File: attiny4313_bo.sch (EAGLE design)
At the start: 11 parts, among them J1 AVR_SPI_PRG_6NS, Y1 16MHz

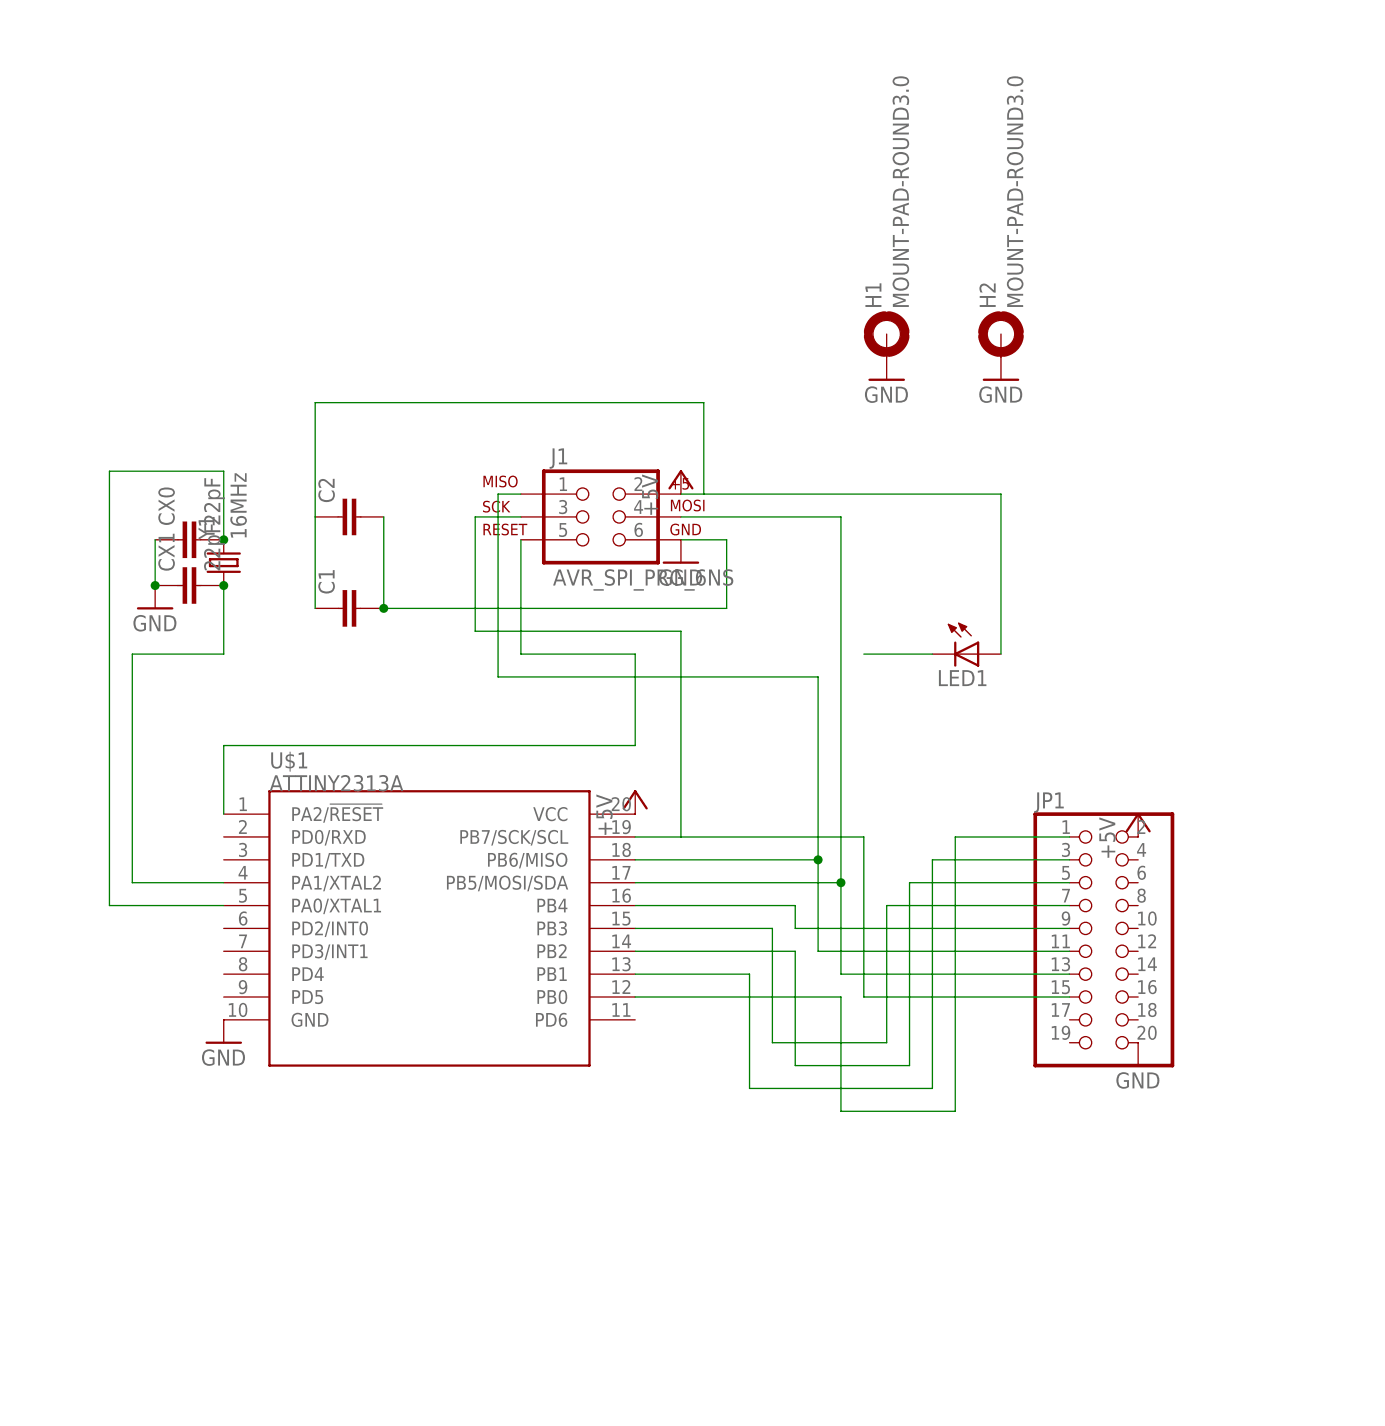
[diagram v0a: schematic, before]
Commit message: signals v1, probably bad
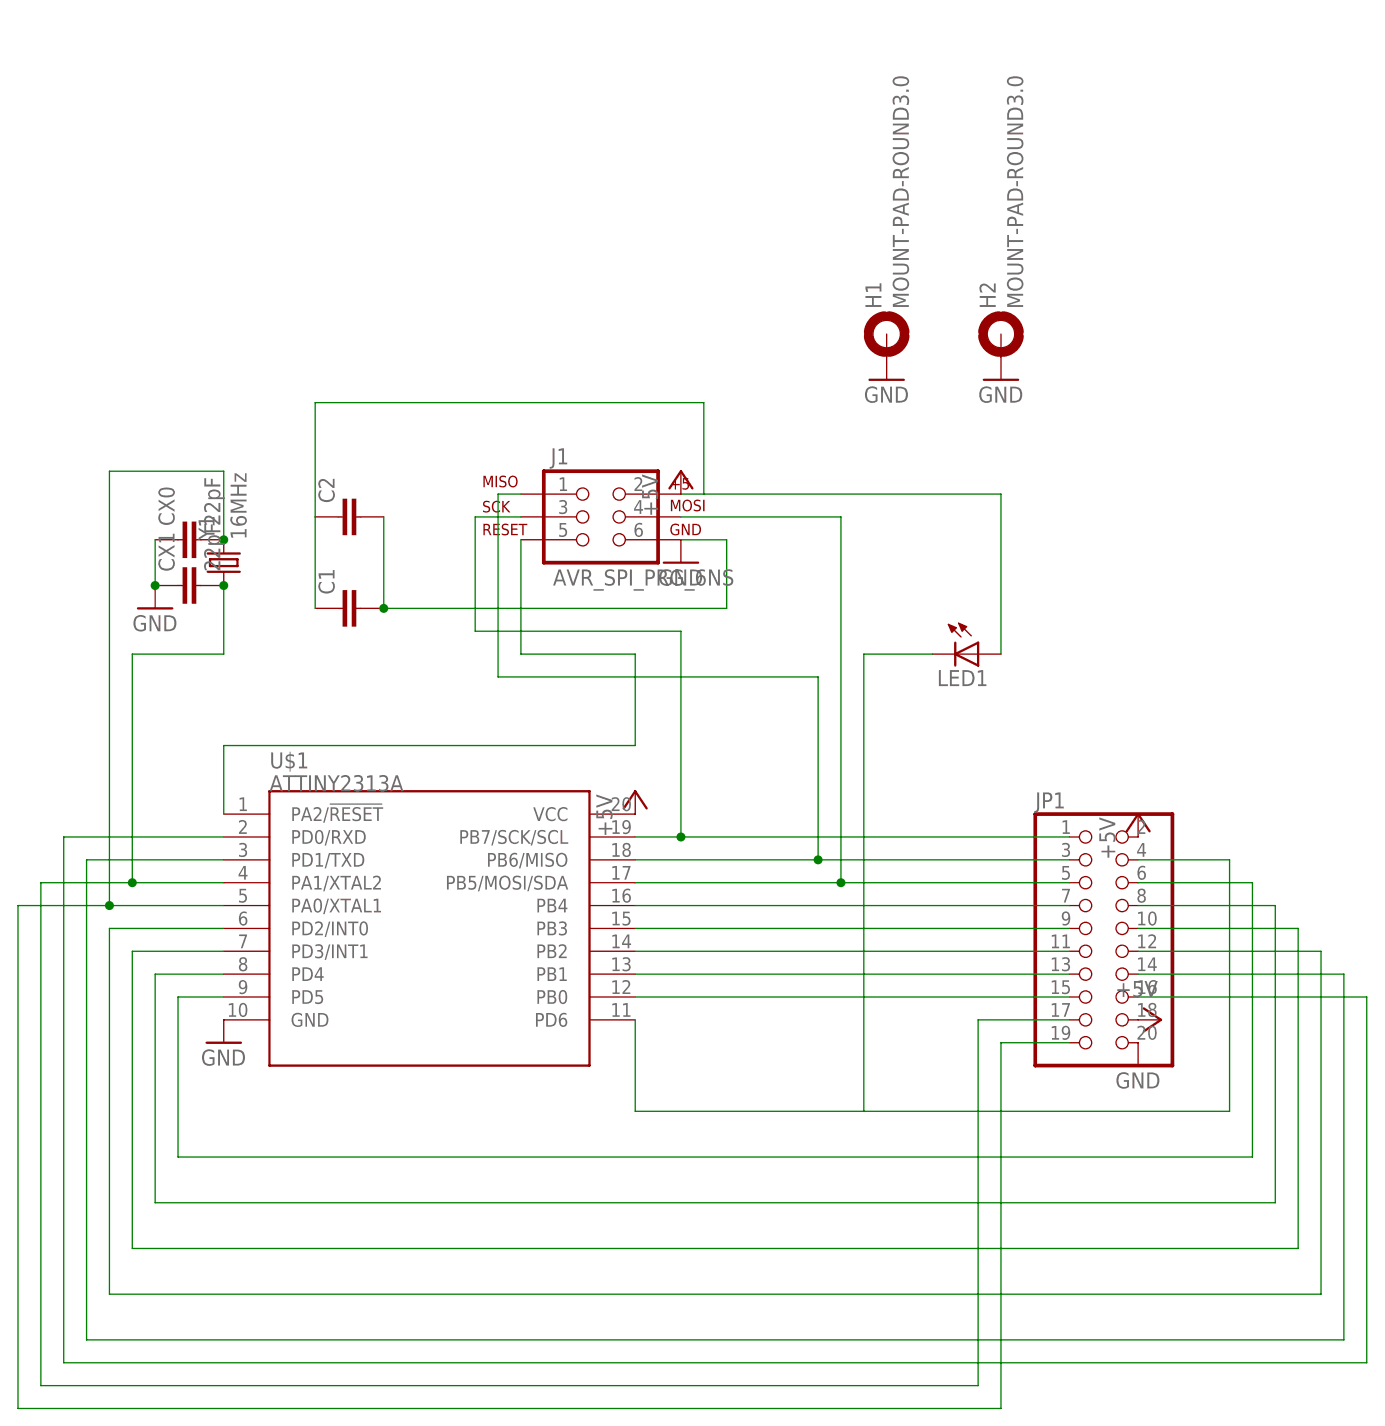
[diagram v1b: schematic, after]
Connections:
- removed net N$1: CX0.2, U$1.PA0/XTAL1, Y1.2
- removed net N$2: LED1.C
- removed net PB0/XTAL1: CX1.2, U$1.PA1/XTAL2, Y1.1
- new net PA0/XTAL1: CX0.2, JP1.19, U$1.PA0/XTAL1, Y1.2
- new net PA1/XTAL2: CX1.2, JP1.17, U$1.PA1/XTAL2, Y1.1
- new net PD0/RDX: JP1.16, U$1.PD0/RXD
- new net PD1/TXD: JP1.14, U$1.PD1/TXD
- new net PD2: JP1.12, U$1.PD2/INT0
- new net PD3: JP1.10, U$1.PD3/INT1
- new net PD4: JP1.8, U$1.PD4
- new net PD5: JP1.6, U$1.PD5
- new net PD6: JP1.4, LED1.C, U$1.PD6
- net +5V: now also JP1.18
- net PB0: now also JP1.15; no longer JP1.1
- net PB1: now also JP1.13; no longer JP1.3
- net PB2: now also JP1.11; no longer JP1.5
- net PB3: now also JP1.9; no longer JP1.7
- net PB4: now also JP1.7; no longer JP1.9
- net PB5/MOSI: now also JP1.5; no longer JP1.13
- net PB6/MISO: now also JP1.3; no longer JP1.11
- net PB7/SCL: now also JP1.1; no longer JP1.15

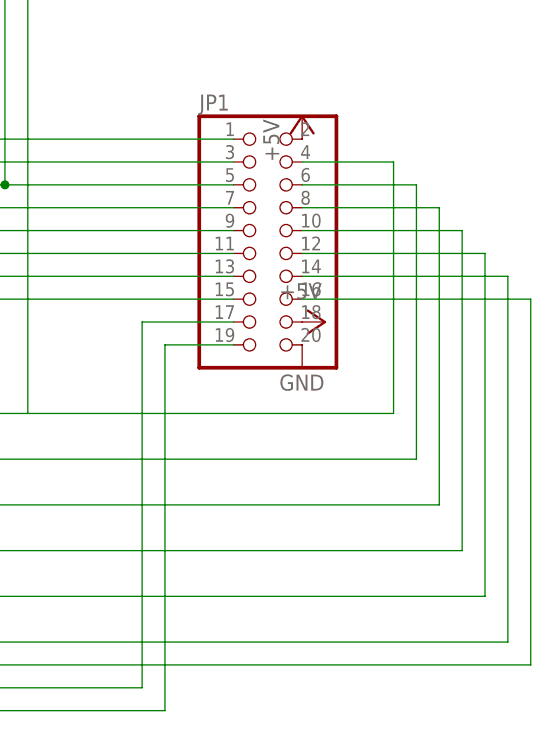
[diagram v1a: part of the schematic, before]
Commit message: pin identifiers
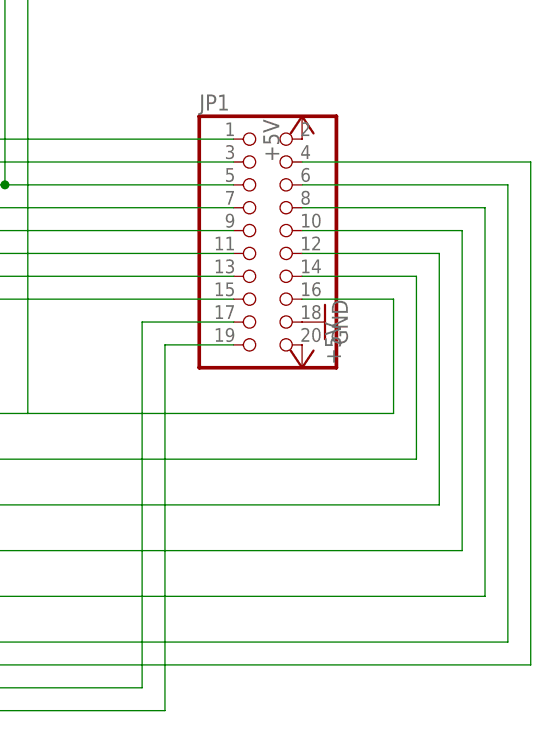
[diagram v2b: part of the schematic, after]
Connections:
- net +5V: now also JP1.20; no longer JP1.18
- net GND: now also JP1.18; no longer JP1.20
- net PD0/RDX: now also JP1.4; no longer JP1.16
- net PD1/TXD: now also JP1.6; no longer JP1.14
- net PD2: now also JP1.8; no longer JP1.12
- net PD4: now also JP1.12; no longer JP1.8
- net PD5: now also JP1.14; no longer JP1.6
- net PD6: now also JP1.16; no longer JP1.4
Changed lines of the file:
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@@
 <part name="P+2" library="supply1" deviceset="+5V" device=""/>
 <part name="JP1" library="pinhead" deviceset="PINHD-2X10" device=""/>
+<part name="P+3" library="supply1" deviceset="+5V" device=""/>
 <part name="GND2" library="supply1" deviceset="GND" device=""/>
-<part name="P+3" library="supply1" deviceset="+5V" device=""/>
 </parts>
 <sheets>
@@
 <instance part="P+2" gate="1" x="127" y="73.66"/>
 <instance part="JP1" gate="A" x="121.92" y="60.96"/>
-<instance part="GND2" gate="1" x="127" y="45.72"/>
-<instance part="P+3" gate="1" x="129.54" y="50.8" rot="R270"/>
+<instance part="P+3" gate="1" x="127" y="45.72" rot="R180"/>
+<instance part="GND2" gate="1" x="129.54" y="50.8" rot="R90"/>
 </instances>
 <busses>
@@
 </segment>
 <segment>
-<pinref part="JP1" gate="A" pin="20"/>
+<pinref part="JP1" gate="A" pin="18"/>
 <pinref part="GND2" gate="1" pin="GND"/>
 </segment>
@@
 </segment>
 <segment>
-<pinref part="JP1" gate="A" pin="18"/>
+<pinref part="JP1" gate="A" pin="20"/>
 <pinref part="P+3" gate="1" pin="+5V"/>
 </segment>
@@
 <segment>
 <wire x1="7.62" y1="12.7" x2="152.4" y2="12.7" width="0.1524" layer="91"/>
-<wire x1="152.4" y1="12.7" x2="152.4" y2="53.34" width="0.1524" layer="91"/>
-<pinref part="JP1" gate="A" pin="16"/>
-<wire x1="152.4" y1="53.34" x2="127" y2="53.34" width="0.1524" layer="91"/>
+<wire x1="152.4" y1="12.7" x2="152.4" y2="68.58" width="0.1524" layer="91"/>
 <wire x1="7.62" y1="12.7" x2="7.62" y2="71.12" width="0.1524" layer="91"/>
 <pinref part="U$1" gate="G$1" pin="PD0/RXD"/>
 <wire x1="7.62" y1="71.12" x2="25.4" y2="71.12" width="0.1524" layer="91"/>
+<pinref part="JP1" gate="A" pin="4"/>
+<wire x1="152.4" y1="68.58" x2="127" y2="68.58" width="0.1524" layer="91"/>
 </segment>
 </net>
@@
 <segment>
 <wire x1="10.16" y1="15.24" x2="149.86" y2="15.24" width="0.1524" layer="91"/>
-<wire x1="149.86" y1="15.24" x2="149.86" y2="55.88" width="0.1524" layer="91"/>
-<pinref part="JP1" gate="A" pin="14"/>
-<wire x1="149.86" y1="55.88" x2="127" y2="55.88" width="0.1524" layer="91"/>
+<wire x1="149.86" y1="15.24" x2="149.86" y2="66.04" width="0.1524" layer="91"/>
 <pinref part="U$1" gate="G$1" pin="PD1/TXD"/>
 <wire x1="25.4" y1="68.58" x2="10.16" y2="68.58" width="0.1524" layer="91"/>
 <wire x1="10.16" y1="15.24" x2="10.16" y2="68.58" width="0.1524" layer="91"/>
+<pinref part="JP1" gate="A" pin="6"/>
+<wire x1="127" y1="66.04" x2="149.86" y2="66.04" width="0.1524" layer="91"/>
 </segment>
 </net>
@@
 <wire x1="71.12" y1="40.64" x2="96.52" y2="40.64" width="0.1524" layer="91"/>
 <wire x1="96.52" y1="40.64" x2="137.16" y2="40.64" width="0.1524" layer="91"/>
-<wire x1="137.16" y1="40.64" x2="137.16" y2="68.58" width="0.1524" layer="91"/>
-<pinref part="JP1" gate="A" pin="4"/>
-<wire x1="137.16" y1="68.58" x2="127" y2="68.58" width="0.1524" layer="91"/>
+<wire x1="137.16" y1="40.64" x2="137.16" y2="53.34" width="0.1524" layer="91"/>
 <pinref part="LED1" gate="G$1" pin="C"/>
 <wire x1="96.52" y1="91.44" x2="104.14" y2="91.44" width="0.1524" layer="91"/>
 <wire x1="96.52" y1="91.44" x2="96.52" y2="40.64" width="0.1524" layer="91"/>
+<pinref part="JP1" gate="A" pin="16"/>
+<wire x1="127" y1="53.34" x2="137.16" y2="53.34" width="0.1524" layer="91"/>
 </segment>
 </net>
@@
 <wire x1="20.32" y1="53.34" x2="20.32" y2="35.56" width="0.1524" layer="91"/>
 <wire x1="20.32" y1="35.56" x2="139.7" y2="35.56" width="0.1524" layer="91"/>
-<wire x1="139.7" y1="35.56" x2="139.7" y2="66.04" width="0.1524" layer="91"/>
-<pinref part="JP1" gate="A" pin="6"/>
-<wire x1="139.7" y1="66.04" x2="127" y2="66.04" width="0.1524" layer="91"/>
+<wire x1="139.7" y1="35.56" x2="139.7" y2="55.88" width="0.1524" layer="91"/>
+<pinref part="JP1" gate="A" pin="14"/>
+<wire x1="139.7" y1="55.88" x2="127" y2="55.88" width="0.1524" layer="91"/>
 </segment>
 </net>
@@
 <wire x1="17.78" y1="55.88" x2="17.78" y2="30.48" width="0.1524" layer="91"/>
 <wire x1="17.78" y1="30.48" x2="142.24" y2="30.48" width="0.1524" layer="91"/>
-<wire x1="142.24" y1="30.48" x2="142.24" y2="63.5" width="0.1524" layer="91"/>
-<pinref part="JP1" gate="A" pin="8"/>
-<wire x1="142.24" y1="63.5" x2="127" y2="63.5" width="0.1524" layer="91"/>
+<wire x1="142.24" y1="30.48" x2="142.24" y2="58.42" width="0.1524" layer="91"/>
+<pinref part="JP1" gate="A" pin="12"/>
+<wire x1="127" y1="58.42" x2="142.24" y2="58.42" width="0.1524" layer="91"/>
 </segment>
 </net>
@@
 <wire x1="12.7" y1="60.96" x2="12.7" y2="20.32" width="0.1524" layer="91"/>
 <wire x1="12.7" y1="20.32" x2="147.32" y2="20.32" width="0.1524" layer="91"/>
-<wire x1="147.32" y1="20.32" x2="147.32" y2="58.42" width="0.1524" layer="91"/>
-<pinref part="JP1" gate="A" pin="12"/>
-<wire x1="147.32" y1="58.42" x2="127" y2="58.42" width="0.1524" layer="91"/>
-</segment>
-</net>
+<wire x1="147.32" y1="20.32" x2="147.32" y2="63.5" width="0.1524" layer="91"/>
+<pinref part="JP1" gate="A" pin="8"/>
+<wire x1="147.32" y1="63.5" x2="127" y2="63.5" width="0.1524" layer="91"/>
+</segment>
+</net>
